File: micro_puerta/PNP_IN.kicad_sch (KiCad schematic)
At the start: 6 parts, among them U4 LTV-357T, U7 LTV-357T

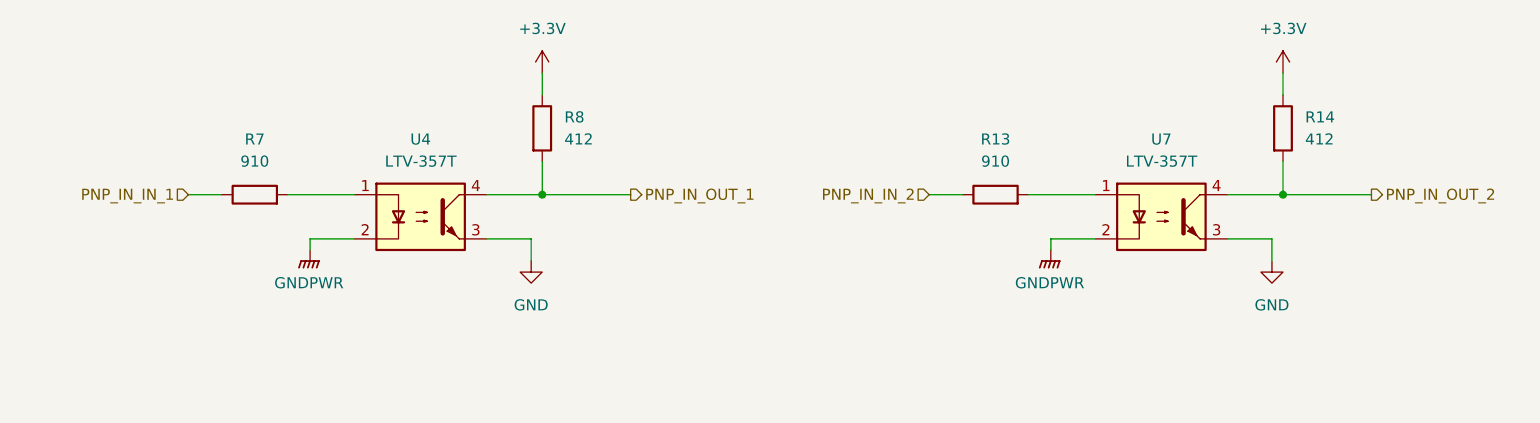
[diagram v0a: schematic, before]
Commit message: Actualizacion 4 de proyecto
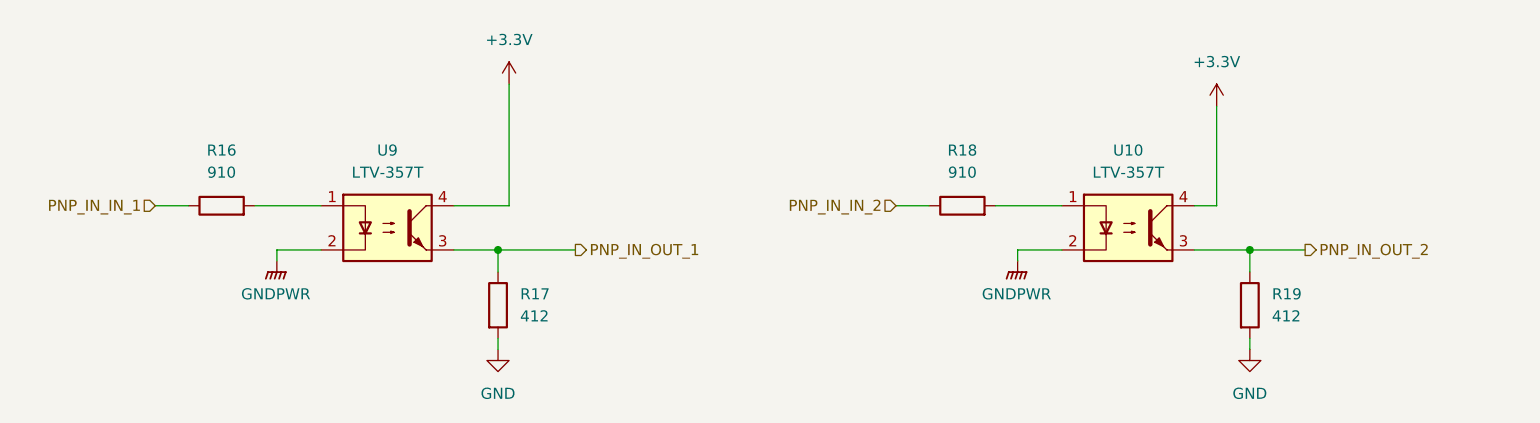
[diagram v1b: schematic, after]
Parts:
- removed R13, R7: 910, symbol Device:R
- removed R14, R8: 412, symbol Device:R
- removed U4, U7: LTV-357T, Package_SO:SO-4_4.4x3.6mm_P2.54mm, symbol Isolator:LTV-357T
- added R16, R18: 910, Resistor_SMD:R_0201_0603Metric, symbol Device:R
- added R17, R19: 412, Resistor_SMD:R_0201_0603Metric, symbol Device:R
- added U10, U9: LTV-357T, Package_SO:SO-4_4.4x3.6mm_P2.54mm, symbol Isolator:LTV-357T
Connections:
- net +3.3V: now also U10.4, U9.4
- net GND: now also R17.2, R19.2
- net GNDPWR: now also U10.2, U9.2
- net PNP_IN_IN_1: now also R16.1
- net PNP_IN_IN_2: now also R18.1
- net PNP_IN_OUT_1: now also R17.1, U9.3
- net PNP_IN_OUT_2: now also R19.1, U10.3
- new net: R18.2, U10.1
- new net: R16.2, U9.1
